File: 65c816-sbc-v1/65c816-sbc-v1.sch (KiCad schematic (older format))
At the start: 56 parts, among them J1 EXPANSION, J2 SIO, J3 VIA_A, J4 VIA_B, J5 power, SW1 RESET, SW2 NMI, U1 W65C816SxP, U10 W65C22SxP, U11 W65C51NxP, U12 74HC138, U15 74HC74, U2 74HC573, U3 74HC245, U4 PAL20L8, U5 PAL20L8, U6 74HC244, U7 74HC244, U8 AS6C4008-55PCN, U9 28C256, X1 28MHz, Y1 1.8432MHz

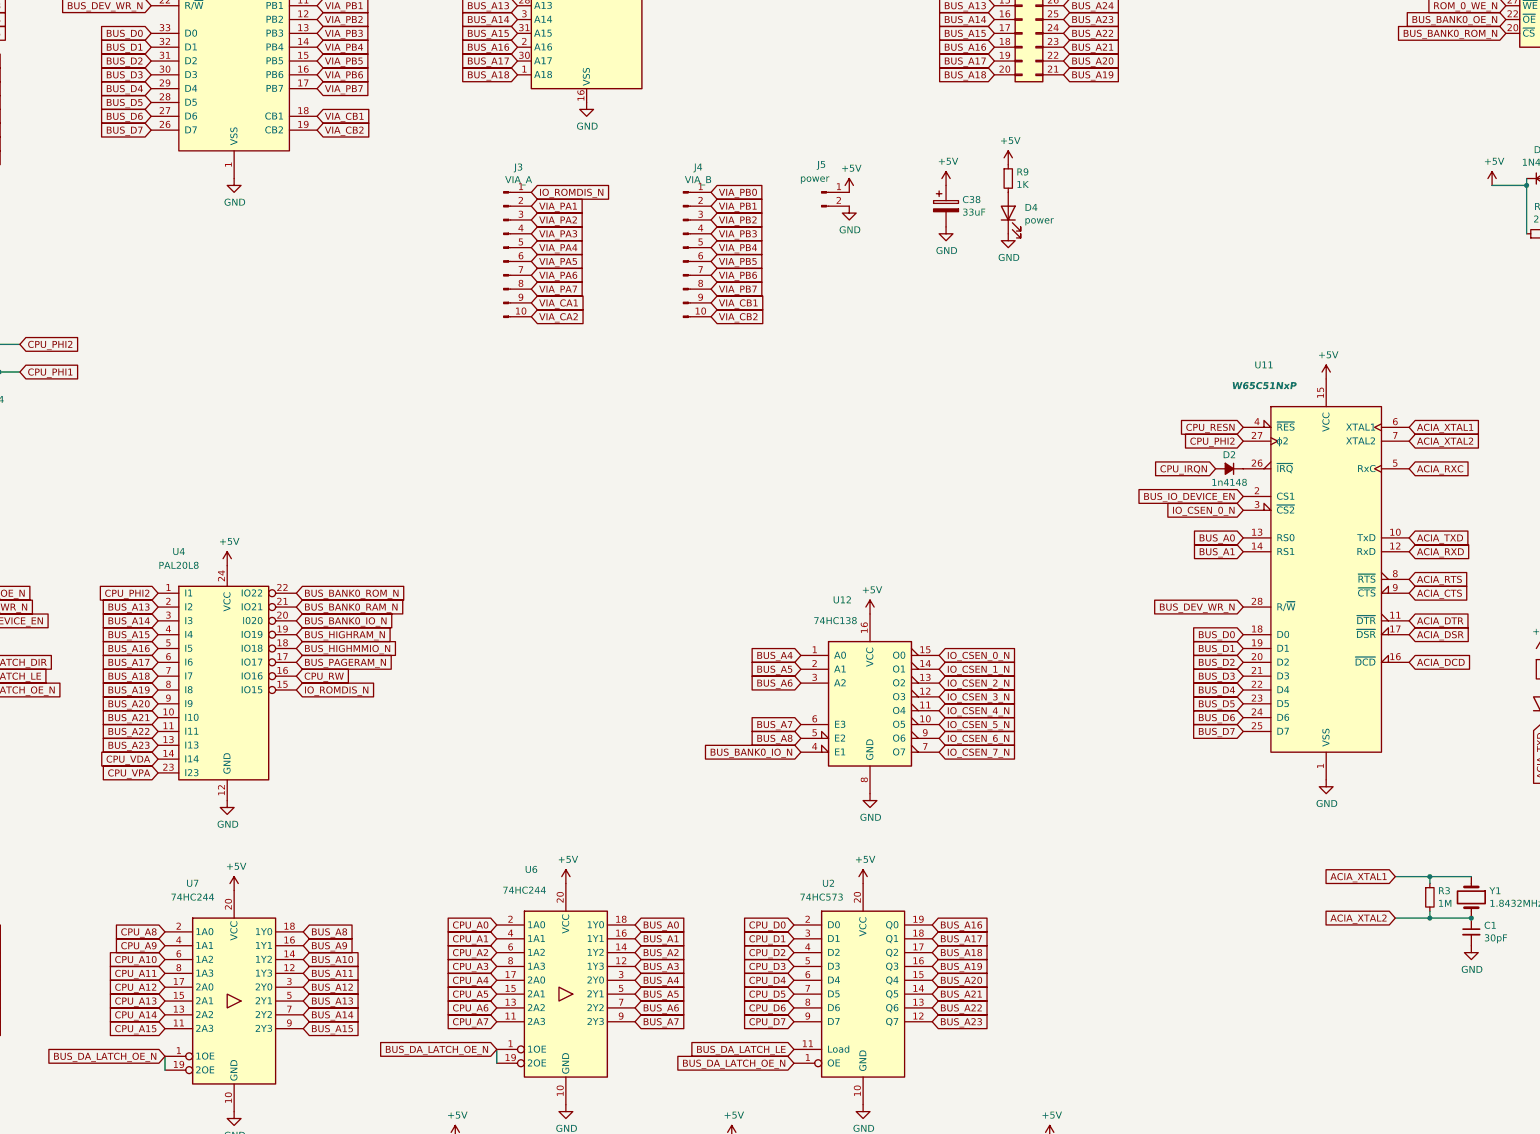
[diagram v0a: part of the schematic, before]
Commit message: more layout inspired changes
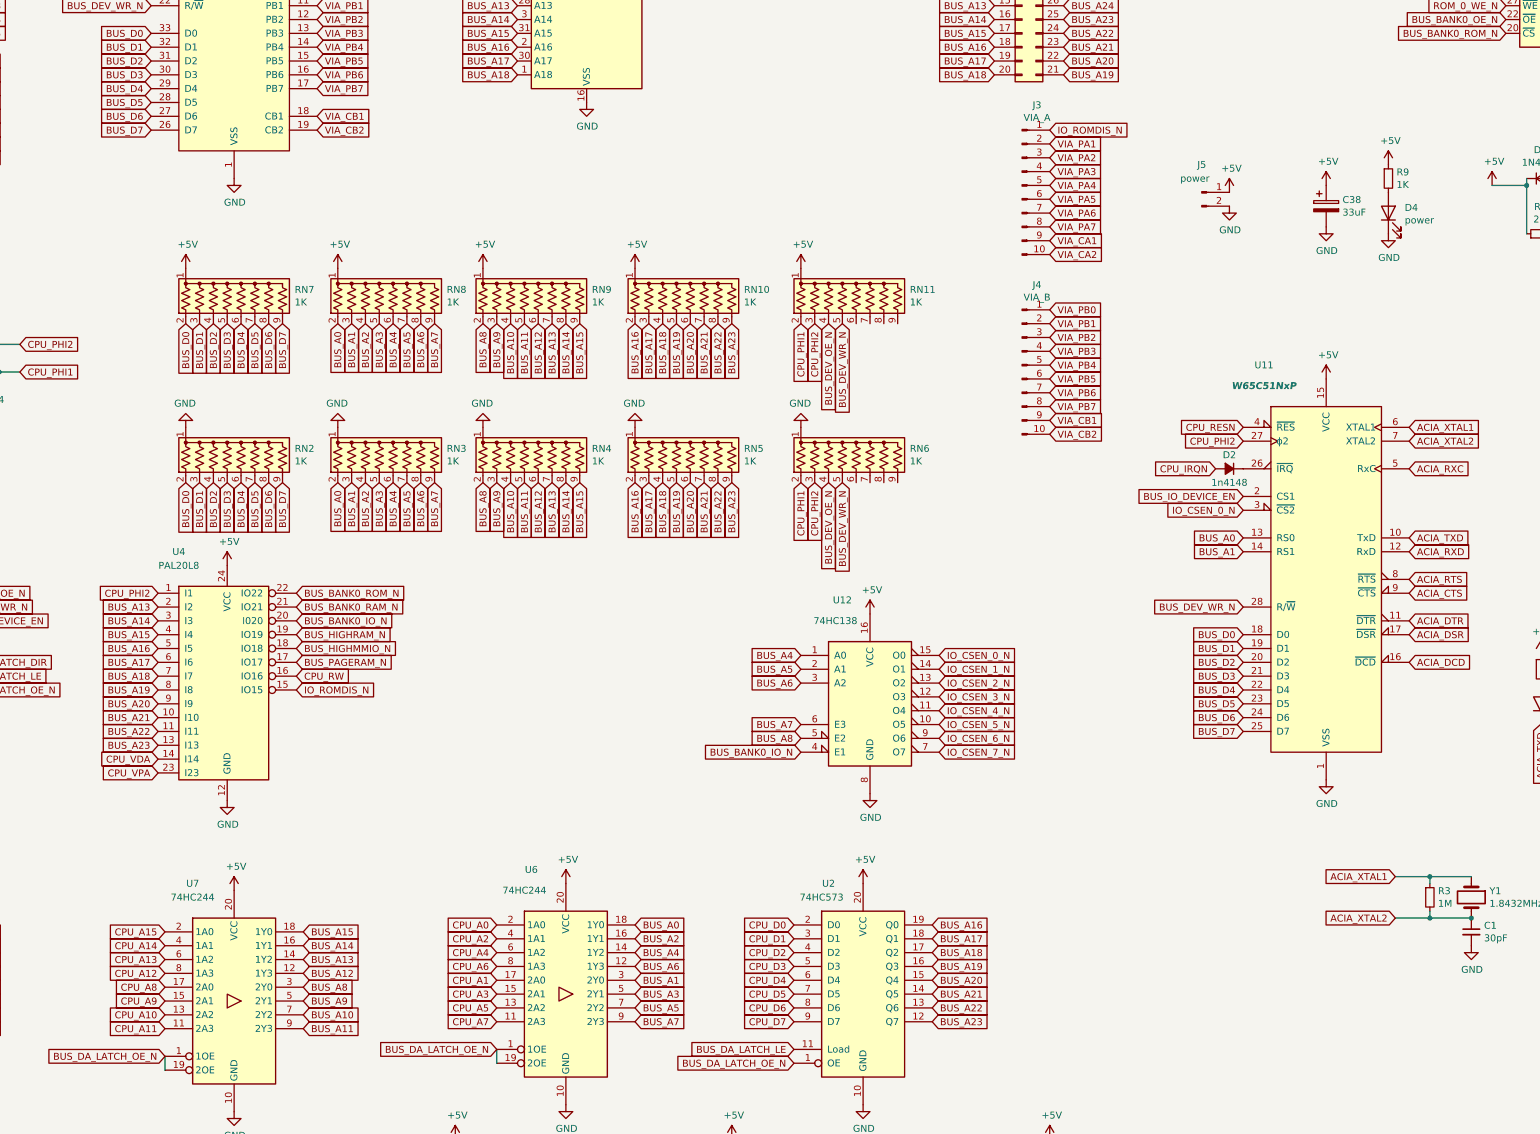
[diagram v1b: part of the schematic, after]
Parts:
- added RN10, RN11, RN2, RN3, RN4, RN5, RN6, RN7, RN8, RN9: 1K, Resistor_THT:R_Array_SIP9, symbol Device:R_Network08_US
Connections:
- net +5V: now also RN10.1 (common), RN11.1 (common), RN7.1 (common), RN8.1 (common), RN9.1 (common)
- net BUS_A0: now also RN3.2 (R1), RN8.2 (R1)
- net BUS_A1: now also U6.3 (2Y0), RN3.3 (R2), RN8.3 (R2); no longer U6.16 (1Y1)
- net BUS_A10: now also U7.7 (2Y2), RN4.4 (R3), RN9.4 (R3); no longer U7.14 (1Y2)
- net BUS_A11: now also U7.9 (2Y3), RN4.5 (R4), RN9.5 (R4); no longer U7.12 (1Y3)
- net BUS_A12: now also U7.12 (1Y3), RN4.6 (R5), RN9.6 (R5); no longer U7.3 (2Y0)
- net BUS_A13: now also U7.14 (1Y2), RN4.7 (R6), RN9.7 (R6); no longer U7.5 (2Y1)
- net BUS_A14: now also U7.16 (1Y1), RN4.8 (R7), RN9.8 (R7); no longer U7.7 (2Y2)
- net BUS_A15: now also U7.18 (1Y0), RN4.9 (R8), RN9.9 (R8); no longer U7.9 (2Y3)
- net BUS_A16: now also RN10.2 (R1), RN5.2 (R1)
- net BUS_A17: now also RN10.3 (R2), RN5.3 (R2)
- net BUS_A18: now also RN10.4 (R3), RN5.4 (R3)
- net BUS_A19: now also RN10.5 (R4), RN5.5 (R4)
- net BUS_A2: now also U6.16 (1Y1), RN3.4 (R3), RN8.4 (R3); no longer U6.14 (1Y2)
- net BUS_A20: now also RN10.6 (R5), RN5.6 (R5)
- net BUS_A21: now also RN10.7 (R6), RN5.7 (R6)
- net BUS_A22: now also RN10.8 (R7), RN5.8 (R7)
- net BUS_A23: now also RN10.9 (R8), RN5.9 (R8)
- net BUS_A3: now also U6.5 (2Y1), RN3.5 (R4), RN8.5 (R4); no longer U6.12 (1Y3)
- net BUS_A4: now also U6.14 (1Y2), RN3.6 (R5), RN8.6 (R5); no longer U6.3 (2Y0)
- net BUS_A5: now also U6.7 (2Y2), RN3.7 (R6), RN8.7 (R6); no longer U6.5 (2Y1)
- net BUS_A6: now also U6.12 (1Y3), RN3.8 (R7), RN8.8 (R7); no longer U6.7 (2Y2)
- net BUS_A7: now also RN3.9 (R8), RN8.9 (R8)
- net BUS_A8: now also U7.3 (2Y0), RN4.2 (R1), RN9.2 (R1); no longer U7.18 (1Y0)
- net BUS_A9: now also U7.5 (2Y1), RN4.3 (R2), RN9.3 (R2); no longer U7.16 (1Y1)
- net BUS_D0: now also RN2.2 (R1), RN7.2 (R1)
- net BUS_D1: now also RN2.3 (R2), RN7.3 (R2)
- net BUS_D2: now also RN2.4 (R3), RN7.4 (R3)
- net BUS_D3: now also RN2.5 (R4), RN7.5 (R4)
- net BUS_D4: now also RN2.6 (R5), RN7.6 (R5)
- net BUS_D5: now also RN2.7 (R6), RN7.7 (R6)
- net BUS_D6: now also RN2.8 (R7), RN7.8 (R7)
- net BUS_D7: now also RN2.9 (R8), RN7.9 (R8)
- net BUS_DEV_OE_N: now also RN11.4 (R3), RN6.4 (R3)
- net BUS_DEV_WR_N: now also RN11.5 (R4), RN6.5 (R4)
- net CPU_A1: now also U6.17 (2A0); no longer U6.4 (1A1)
- net CPU_A10: now also U7.13 (2A2); no longer U7.6 (1A2)
- net CPU_A11: now also U7.11 (2A3); no longer U7.8 (1A3)
- net CPU_A12: now also U7.8 (1A3); no longer U7.17 (2A0)
- net CPU_A13: now also U7.6 (1A2); no longer U7.15 (2A1)
- net CPU_A14: now also U7.4 (1A1); no longer U7.13 (2A2)
- net CPU_A15: now also U7.2 (1A0); no longer U7.11 (2A3)
- net CPU_A2: now also U6.4 (1A1); no longer U6.6 (1A2)
- net CPU_A3: now also U6.15 (2A1); no longer U6.8 (1A3)
- net CPU_A4: now also U6.6 (1A2); no longer U6.17 (2A0)
- net CPU_A5: now also U6.13 (2A2); no longer U6.15 (2A1)
- net CPU_A6: now also U6.8 (1A3); no longer U6.13 (2A2)
- net CPU_A8: now also U7.17 (2A0); no longer U7.2 (1A0)
- net CPU_A9: now also U7.15 (2A1); no longer U7.4 (1A1)
- net CPU_PHI1: now also RN11.2 (R1), RN6.2 (R1)
- net CPU_PHI2: now also RN11.3 (R2), RN6.3 (R2)
- net GND: now also RN2.1 (common), RN3.1 (common), RN4.1 (common), RN5.1 (common), RN6.1 (common)
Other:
- moved on the sheet: C38, D4, J3, J4, J5, R9

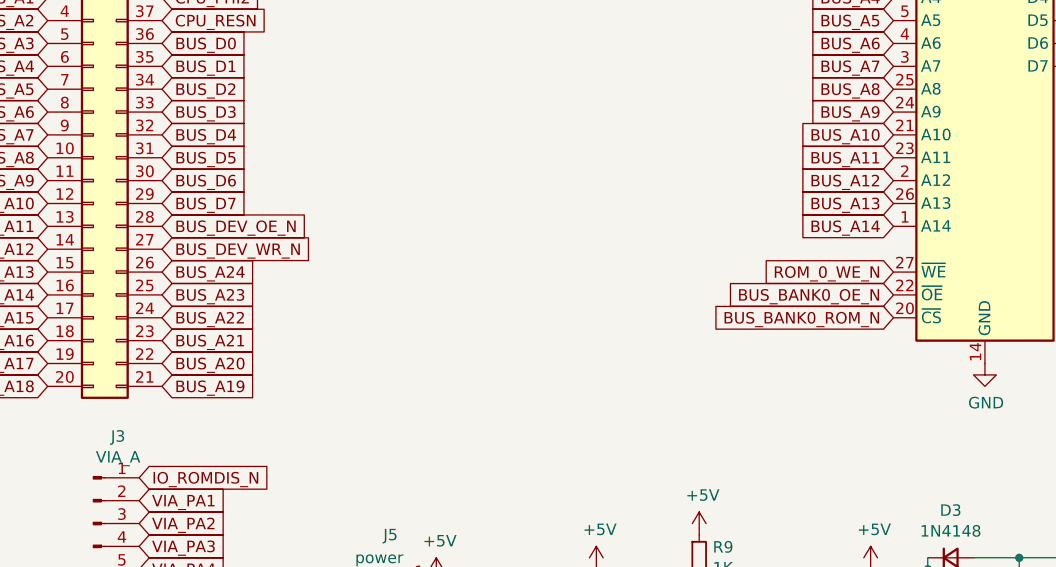
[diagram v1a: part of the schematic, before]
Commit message: another update; i'm not liking how this is working out right now.
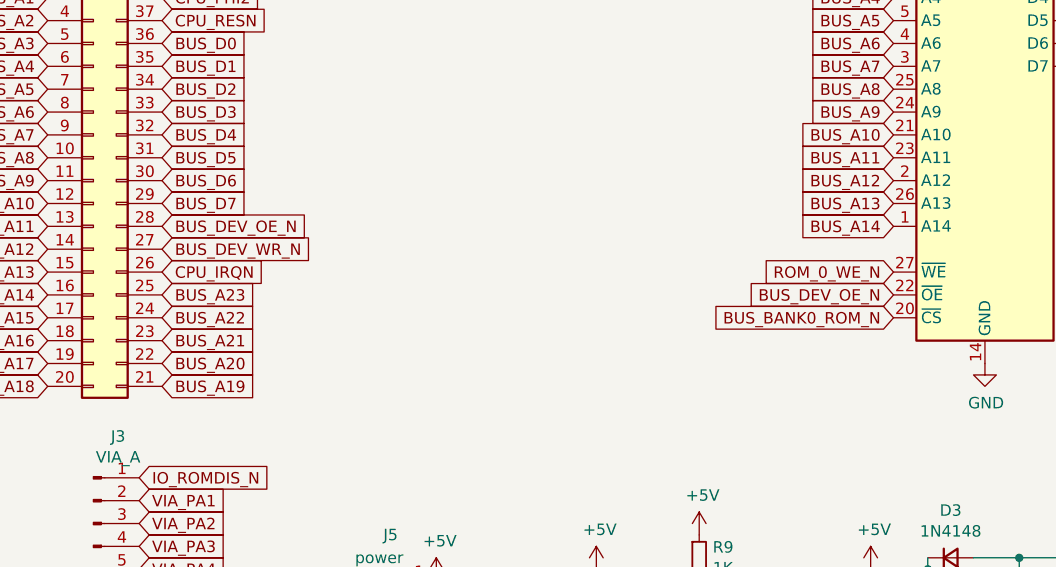
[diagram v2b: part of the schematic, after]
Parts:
- C1, C20, C21, C22, C23, C24, C25, C26, C27, C28, C29, C30, C31, C32, C33, C34, C35, C36, C37: footprint Capacitor_THT:C_Rect_L7.5mm_W6.5mm_P5.00mm -> Capacitor_THT:C_Rect_L4.0mm_W2.5mm_P2.50mm
- C3, C38: footprint Capacitor_THT:CP_Radial_D10.0mm_P7.50mm -> Capacitor_THT:CP_Radial_D6.3mm_P2.50mm
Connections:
- net BUS_A24 is gone; now on net CPU_IRQN: J1.26 (Pin_26)
- net BUS_BANK0_OE_N is gone; now on net BUS_DEV_OE_N: U9.22 (~OE)
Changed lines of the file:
@@
 BUS_BANK0_ROM_N
 Text GLabel 13950 2600 0    50   Input ~ 0
-BUS_BANK0_OE_N
+BUS_DEV_OE_N
 $Comp
 L Device:R_Small R2
@@
 F 0 "C1" H 13792 9246 50  0000 L CNN
 F 1 "30pF" H 13792 9155 50  0000 L CNN
-F 2 "Capacitor_THT:C_Rect_L7.5mm_W6.5mm_P5.00mm" H 13700 9200 50  0001 C CNN
+F 2 "Capacitor_THT:C_Rect_L4.0mm_W2.5mm_P2.50mm" H 13700 9200 50  0001 C CNN
 F 3 "~" H 13700 9200 50  0001 C CNN
 	1    13700 9200
@@
 F 0 "C21" H 10092 10846 50  0000 L CNN
 F 1 "0.1u" H 10092 10755 50  0000 L CNN
-F 2 "Capacitor_THT:C_Rect_L7.5mm_W6.5mm_P5.00mm" H 10000 10800 50  0001 C CNN
+F 2 "Capacitor_THT:C_Rect_L4.0mm_W2.5mm_P2.50mm" H 10000 10800 50  0001 C CNN
 F 3 "~" H 10000 10800 50  0001 C CNN
 	1    10000 10800
@@
 F 0 "C22" H 10442 10846 50  0000 L CNN
 F 1 "0.1u" H 10442 10755 50  0000 L CNN
-F 2 "Capacitor_THT:C_Rect_L7.5mm_W6.5mm_P5.00mm" H 10350 10800 50  0001 C CNN
+F 2 "Capacitor_THT:C_Rect_L4.0mm_W2.5mm_P2.50mm" H 10350 10800 50  0001 C CNN
 F 3 "~" H 10350 10800 50  0001 C CNN
 	1    10350 10800
@@
 F 0 "C23" H 10742 10846 50  0000 L CNN
 F 1 "0.1u" H 10742 10755 50  0000 L CNN
-F 2 "Capacitor_THT:C_Rect_L7.5mm_W6.5mm_P5.00mm" H 10650 10800 50  0001 C CNN
+F 2 "Capacitor_THT:C_Rect_L4.0mm_W2.5mm_P2.50mm" H 10650 10800 50  0001 C CNN
 F 3 "~" H 10650 10800 50  0001 C CNN
 	1    10650 10800
@@
 F 0 "C24" H 11092 10846 50  0000 L CNN
 F 1 "0.1u" H 11092 10755 50  0000 L CNN
-F 2 "Capacitor_THT:C_Rect_L7.5mm_W6.5mm_P5.00mm" H 11000 10800 50  0001 C CNN
+F 2 "Capacitor_THT:C_Rect_L4.0mm_W2.5mm_P2.50mm" H 11000 10800 50  0001 C CNN
 F 3 "~" H 11000 10800 50  0001 C CNN
 	1    11000 10800
@@
 F 0 "C25" H 11442 10846 50  0000 L CNN
 F 1 "0.1u" H 11442 10755 50  0000 L CNN
-F 2 "Capacitor_THT:C_Rect_L7.5mm_W6.5mm_P5.00mm" H 11350 10800 50  0001 C CNN
+F 2 "Capacitor_THT:C_Rect_L4.0mm_W2.5mm_P2.50mm" H 11350 10800 50  0001 C CNN
 F 3 "~" H 11350 10800 50  0001 C CNN
 	1    11350 10800
@@
 F 0 "C20" H 9792 10846 50  0000 L CNN
 F 1 "0.1u" H 9792 10755 50  0000 L CNN
-F 2 "Capacitor_THT:C_Rect_L7.5mm_W6.5mm_P5.00mm" H 9700 10800 50  0001 C CNN
+F 2 "Capacitor_THT:C_Rect_L4.0mm_W2.5mm_P2.50mm" H 9700 10800 50  0001 C CNN
 F 3 "~" H 9700 10800 50  0001 C CNN
 	1    9700 10800
@@
 F 0 "C26" H 7592 10846 50  0000 L CNN
 F 1 "0.1u" H 7592 10755 50  0000 L CNN
-F 2 "Capacitor_THT:C_Rect_L7.5mm_W6.5mm_P5.00mm" H 7500 10800 50  0001 C CNN
+F 2 "Capacitor_THT:C_Rect_L4.0mm_W2.5mm_P2.50mm" H 7500 10800 50  0001 C CNN
 F 3 "~" H 7500 10800 50  0001 C CNN
 	1    7500 10800
@@
 F 0 "C27" H 7892 10846 50  0000 L CNN
 F 1 "0.1u" H 7892 10755 50  0000 L CNN
-F 2 "Capacitor_THT:C_Rect_L7.5mm_W6.5mm_P5.00mm" H 7800 10800 50  0001 C CNN
+F 2 "Capacitor_THT:C_Rect_L4.0mm_W2.5mm_P2.50mm" H 7800 10800 50  0001 C CNN
 F 3 "~" H 7800 10800 50  0001 C CNN
 	1    7800 10800
@@
 F 0 "C28" H 8142 10846 50  0000 L CNN
 F 1 "0.1u" H 8142 10755 50  0000 L CNN
-F 2 "Capacitor_THT:C_Rect_L7.5mm_W6.5mm_P5.00mm" H 8050 10800 50  0001 C CNN
+F 2 "Capacitor_THT:C_Rect_L4.0mm_W2.5mm_P2.50mm" H 8050 10800 50  0001 C CNN
 F 3 "~" H 8050 10800 50  0001 C CNN
 	1    8050 10800
@@
 F 0 "C29" H 8442 10846 50  0000 L CNN
 F 1 "0.1u" H 8442 10755 50  0000 L CNN
-F 2 "Capacitor_THT:C_Rect_L7.5mm_W6.5mm_P5.00mm" H 8350 10800 50  0001 C CNN
+F 2 "Capacitor_THT:C_Rect_L4.0mm_W2.5mm_P2.50mm" H 8350 10800 50  0001 C CNN
 F 3 "~" H 8350 10800 50  0001 C CNN
 	1    8350 10800
@@
 F 0 "C30" H 8742 10846 50  0000 L CNN
 F 1 "0.1u" H 8742 10755 50  0000 L CNN
-F 2 "Capacitor_THT:C_Rect_L7.5mm_W6.5mm_P5.00mm" H 8650 10800 50  0001 C CNN
+F 2 "Capacitor_THT:C_Rect_L4.0mm_W2.5mm_P2.50mm" H 8650 10800 50  0001 C CNN
 F 3 "~" H 8650 10800 50  0001 C CNN
 	1    8650 10800
@@
 F 0 "C31" H 9042 10846 50  0000 L CNN
 F 1 "0.1u" H 9042 10755 50  0000 L CNN
-F 2 "Capacitor_THT:C_Rect_L7.5mm_W6.5mm_P5.00mm" H 8950 10800 50  0001 C CNN
+F 2 "Capacitor_THT:C_Rect_L4.0mm_W2.5mm_P2.50mm" H 8950 10800 50  0001 C CNN
 F 3 "~" H 8950 10800 50  0001 C CNN
 	1    8950 10800
@@
 Text GLabel 10750 2600 2    50   Input ~ 0
 BUS_A23
-Text GLabel 10750 2500 2    50   Input ~ 0
-BUS_A24
 Text GLabel 10750 1200 2    50   Input ~ 0
 CPU_PHI1
@@
 F 0 "C32" H 5592 10846 50  0000 L CNN
 F 1 "0.1u" H 5592 10755 50  0000 L CNN
-F 2 "Capacitor_THT:C_Rect_L7.5mm_W6.5mm_P5.00mm" H 5500 10800 50  0001 C CNN
+F 2 "Capacitor_THT:C_Rect_L4.0mm_W2.5mm_P2.50mm" H 5500 10800 50  0001 C CNN
 F 3 "~" H 5500 10800 50  0001 C CNN
 	1    5500 10800
@@
 F 0 "C33" H 5892 10846 50  0000 L CNN
 F 1 "0.1u" H 5892 10755 50  0000 L CNN
-F 2 "Capacitor_THT:C_Rect_L7.5mm_W6.5mm_P5.00mm" H 5800 10800 50  0001 C CNN
+F 2 "Capacitor_THT:C_Rect_L4.0mm_W2.5mm_P2.50mm" H 5800 10800 50  0001 C CNN
 F 3 "~" H 5800 10800 50  0001 C CNN
 	1    5800 10800
@@
 F 0 "C34" H 6142 10846 50  0000 L CNN
 F 1 "0.1u" H 6142 10755 50  0000 L CNN
-F 2 "Capacitor_THT:C_Rect_L7.5mm_W6.5mm_P5.00mm" H 6050 10800 50  0001 C CNN
+F 2 "Capacitor_THT:C_Rect_L4.0mm_W2.5mm_P2.50mm" H 6050 10800 50  0001 C CNN
 F 3 "~" H 6050 10800 50  0001 C CNN
 	1    6050 10800
@@
 F 0 "C35" H 6442 10846 50  0000 L CNN
 F 1 "0.1u" H 6442 10755 50  0000 L CNN
-F 2 "Capacitor_THT:C_Rect_L7.5mm_W6.5mm_P5.00mm" H 6350 10800 50  0001 C CNN
+F 2 "Capacitor_THT:C_Rect_L4.0mm_W2.5mm_P2.50mm" H 6350 10800 50  0001 C CNN
 F 3 "~" H 6350 10800 50  0001 C CNN
 	1    6350 10800
@@
 F 0 "C36" H 6742 10846 50  0000 L CNN
 F 1 "0.1u" H 6742 10755 50  0000 L CNN
-F 2 "Capacitor_THT:C_Rect_L7.5mm_W6.5mm_P5.00mm" H 6650 10800 50  0001 C CNN
+F 2 "Capacitor_THT:C_Rect_L4.0mm_W2.5mm_P2.50mm" H 6650 10800 50  0001 C CNN
 F 3 "~" H 6650 10800 50  0001 C CNN
 	1    6650 10800
@@
 F 0 "C37" H 7042 10846 50  0000 L CNN
 F 1 "0.1u" H 7042 10755 50  0000 L CNN
-F 2 "Capacitor_THT:C_Rect_L7.5mm_W6.5mm_P5.00mm" H 6950 10800 50  0001 C CNN
+F 2 "Capacitor_THT:C_Rect_L4.0mm_W2.5mm_P2.50mm" H 6950 10800 50  0001 C CNN
 F 3 "~" H 6950 10800 50  0001 C CNN
 	1    6950 10800
@@
 F 0 "C38" H 12768 3996 50  0000 L CNN
 F 1 "33uF" H 12768 3905 50  0000 L CNN
-F 2 "Capacitor_THT:CP_Radial_D10.0mm_P7.50mm" H 12688 3800 50  0001 C CNN
+F 2 "Capacitor_THT:CP_Radial_D6.3mm_P2.50mm" H 12688 3800 50  0001 C CNN
 F 3 "~" H 12650 3950 50  0001 C CNN
 	1    12650 3950
@@
 F 0 "C3" H 15268 3996 50  0000 L CNN
 F 1 "1uF" H 15268 3905 50  0000 L CNN
-F 2 "Capacitor_THT:CP_Radial_D10.0mm_P7.50mm" H 15188 3800 50  0001 C CNN
+F 2 "Capacitor_THT:CP_Radial_D6.3mm_P2.50mm" H 15188 3800 50  0001 C CNN
 F 3 "~" H 15150 3950 50  0001 C CNN
 	1    15150 3950
@@
 Text GLabel 4250 9600 0    50   Input ~ 0
 CPU_A8
+Text GLabel 10750 2500 2    50   Input ~ 0
+CPU_IRQN
 $EndSCHEMATC
